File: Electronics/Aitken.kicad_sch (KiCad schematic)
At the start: 0 parts

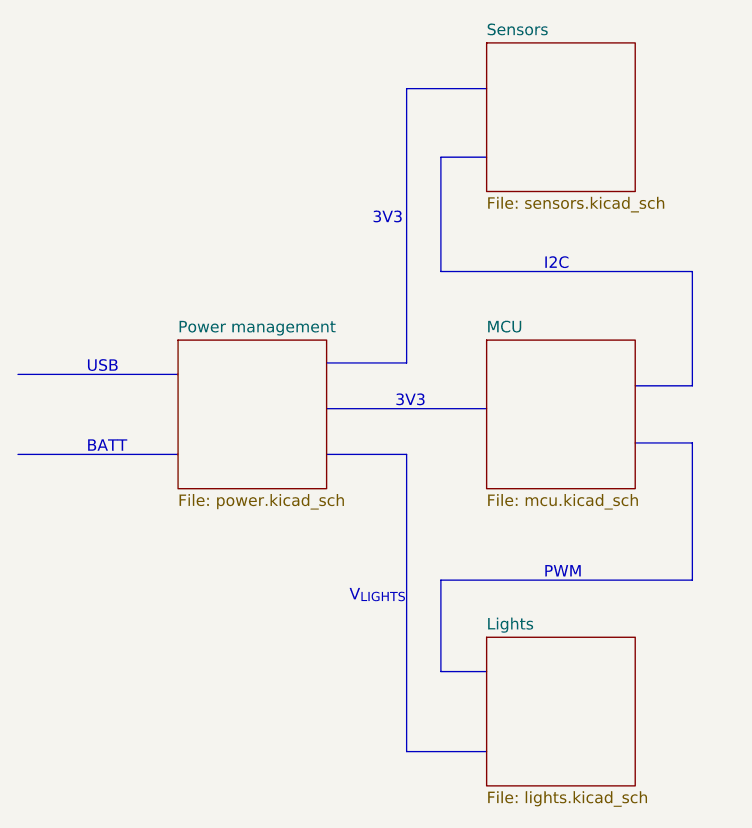
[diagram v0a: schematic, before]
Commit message: Power and lights update
Changed STUSB4500 + BQ25895 to MP2722. Changed Lights power supply, now it's split up to 3 LED drivers - KTD2801 as 10s1p. Added fuses to each battery. Added ESD protection. Fixed CHIP_EN pin name on ESP32-C3 and pull-up resistor on I2C lines.
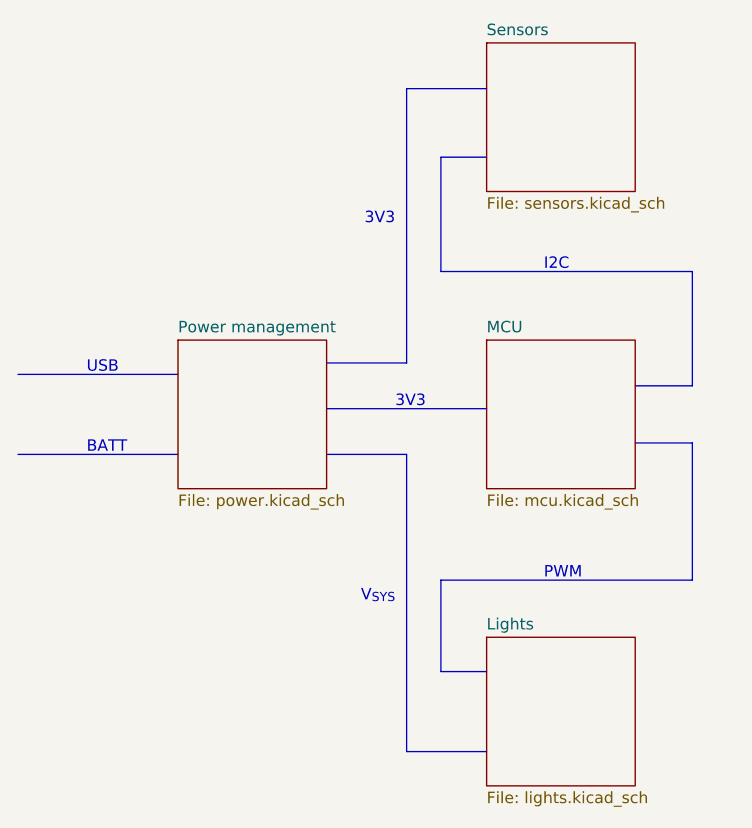
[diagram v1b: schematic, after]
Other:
- note added: "V_{SYS}"
- note removed: "V_{LIGHTS}"
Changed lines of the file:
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@@
     (stroke (width 0) (type default))
   )
-  (text "V_{LIGHTS}" (at 138.43 119.38 0)
+  (text "V_{SYS}" (at 139.7 119.38 0)
     (effects (font (size 1.27 1.27) (color 255 0 0 1)) (justify left bottom))
   )
@@
     (effects (font (size 1.27 1.27) (color 255 0 0 1)) (justify left bottom))
   )
-  (text "3V3" (at 140.97 77.47 0)
-    (effects (font (size 1.27 1.27) (color 255 0 0 1)) (justify left bottom))
+  (text "3V3" (at 143.51 77.47 0)
+    (effects (font (size 1.27 1.27) (color 255 0 0 1)) (justify right bottom))
   )
   (text "I2C" (at 160.02 82.55 0)
